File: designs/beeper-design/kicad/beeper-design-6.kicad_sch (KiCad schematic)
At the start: 23 parts, among them U3 BQ51003YFPR, U5 FH19C-6S-0.5SH(10)

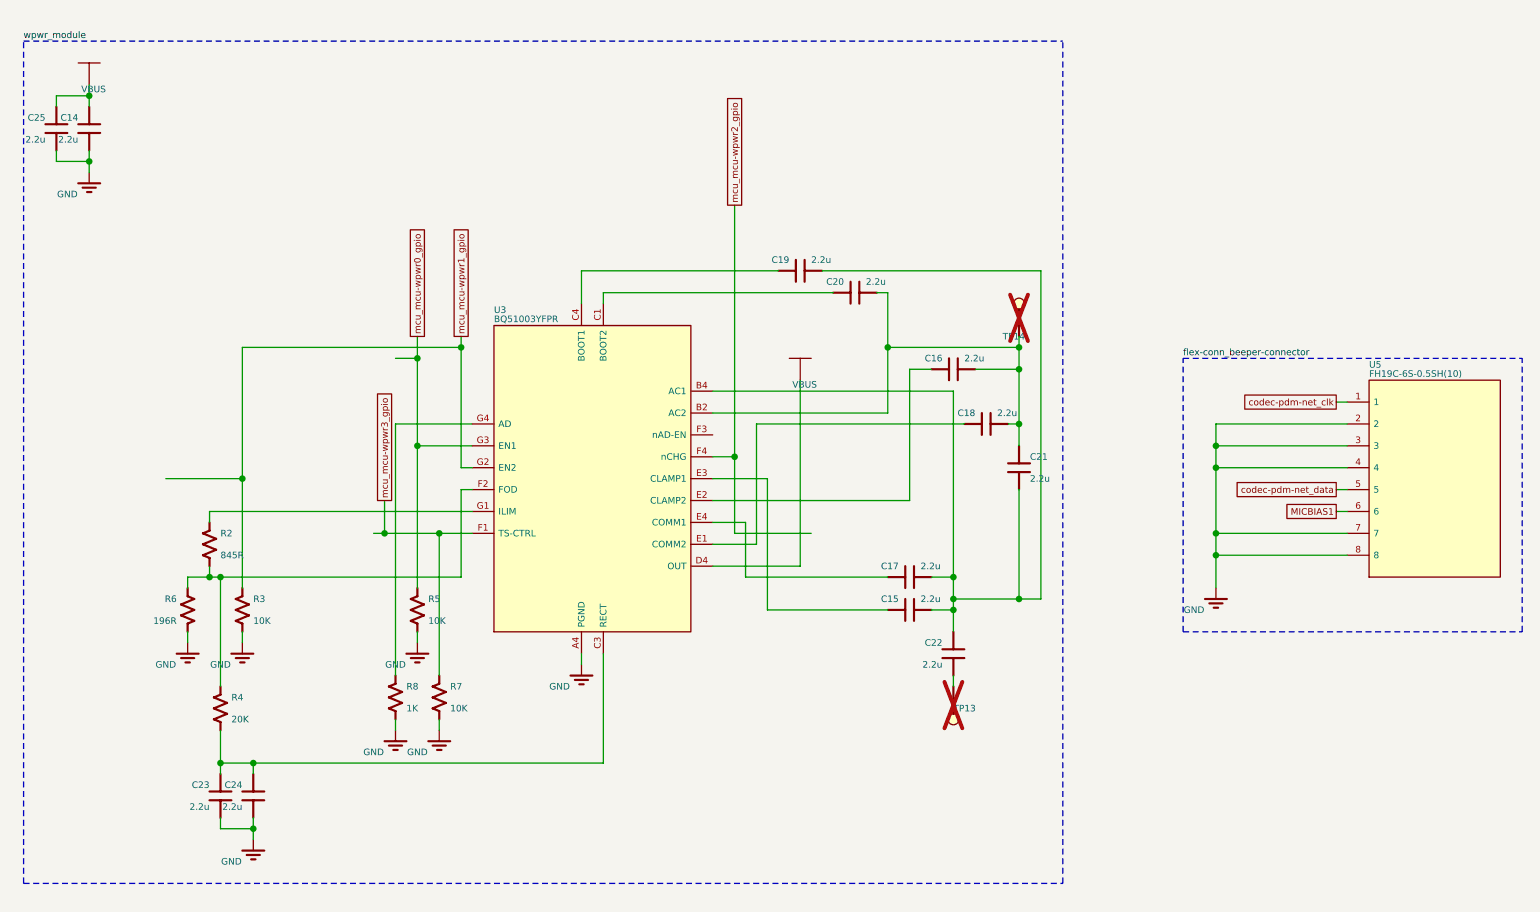
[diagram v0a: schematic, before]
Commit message: new export
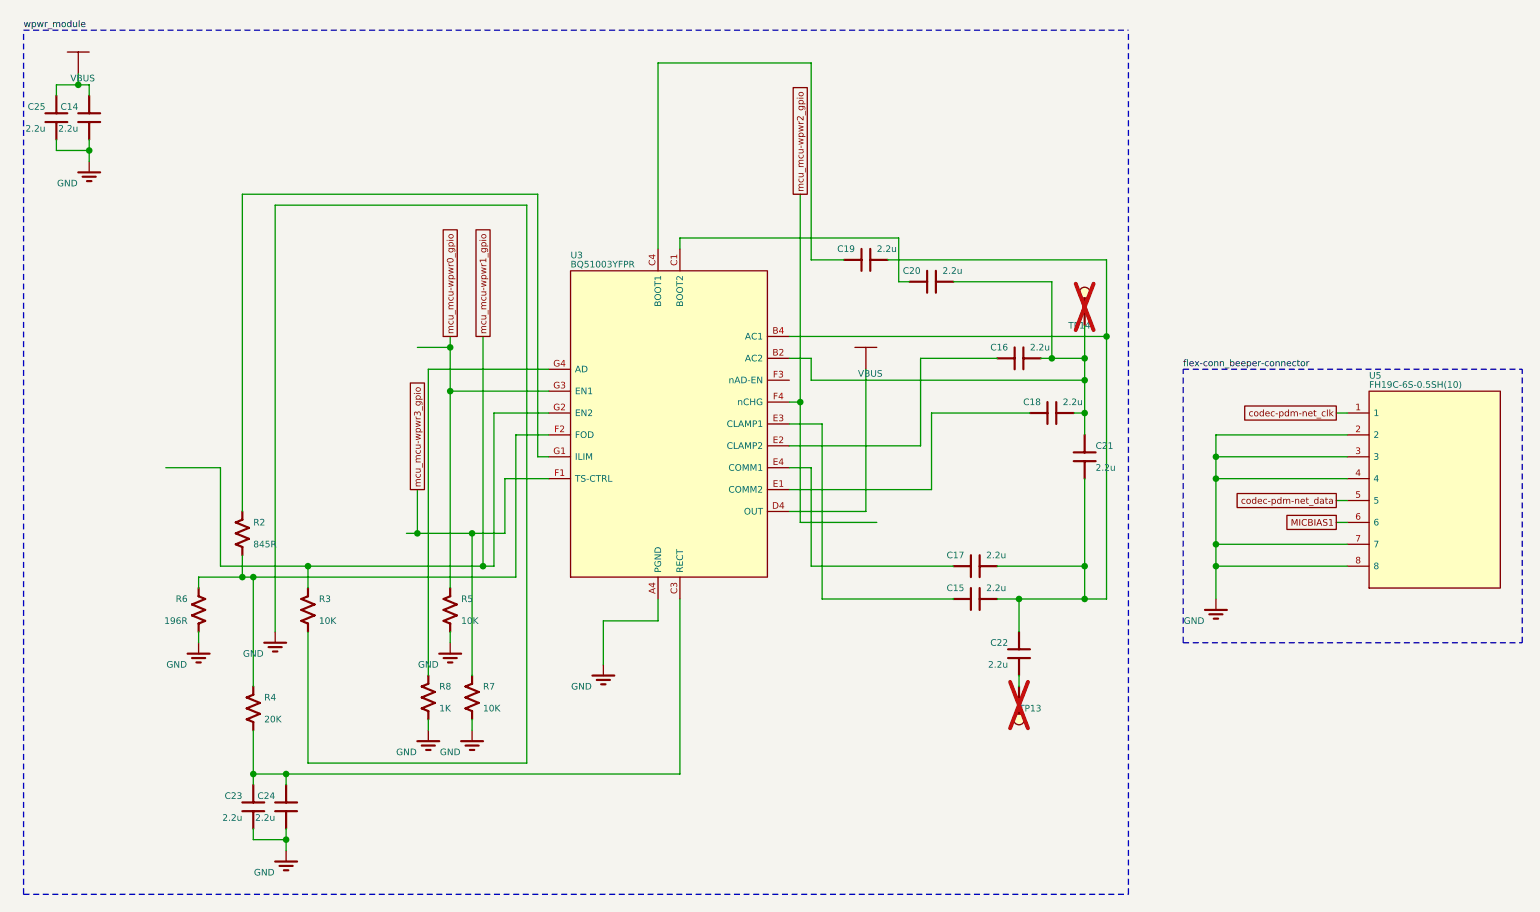
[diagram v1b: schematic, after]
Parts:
- removed C14: 2.2u, beeper-design:Pkg0201_2, symbol C335106
- removed C15: 2.2u, beeper-design:Pkg0201_51, symbol C335106_35
- removed C16: 2.2u, beeper-design:Pkg0201_12, symbol C335106_10
- removed C17: 2.2u, beeper-design:Pkg0201_25, symbol C335106_18
- removed C18: 2.2u, beeper-design:Pkg0201_37, symbol C335106_26
- removed C19: 2.2u, beeper-design:Pkg0201_49, symbol C335106_33
- removed C20: 2.2u, beeper-design:Pkg0201_10, symbol C335106_8
- removed C21: 2.2u, beeper-design:Pkg0201_23, symbol C335106_16
- removed C22: 2.2u, beeper-design:Pkg0201_35, symbol C335106_25
- removed C23: 2.2u, beeper-design:Pkg0201_48, symbol C335106_32
- removed C24: 2.2u, beeper-design:Pkg0201_7, symbol C335106_5
- removed C25: 2.2u, beeper-design:Pkg0201_22, symbol C335106_15
- removed R2: 845R, beeper-design:Pkg0201_15, symbol my_resistor_1
- removed R4: 20K, beeper-design:Pkg0201_41, symbol my_resistor_10
- removed R7: 10K, beeper-design:Pkg0201_26, symbol my_resistor_5
- removed R8: 1K, beeper-design:Pkg0201_38, symbol my_resistor_8
- added C14: 2.2u, beeper-design:Pkg0201, symbol C335106_35
- added C15: 2.2u, beeper-design:Pkg0201_50, symbol C335106_31
- added C16: 2.2u, beeper-design:Pkg0201_9, symbol C335106_7
- added C17: 2.2u, beeper-design:Pkg0201_22, symbol C335106_14
- added C18: 2.2u, beeper-design:Pkg0201_36, symbol C335106_22
- added C19: 2.2u, beeper-design:Pkg0201_49, symbol C335106_30
- added C20: 2.2u, beeper-design:Pkg0201_7, symbol C335106_5
- added C21: 2.2u, beeper-design:Pkg0201_20, symbol C335106_12
- added C22: 2.2u, beeper-design:Pkg0201_33, symbol C335106_20
- added C23: 2.2u, beeper-design:Pkg0201_48, symbol C335106_29
- added C24: 2.2u, beeper-design:Pkg0201_6, symbol C335106_4
- added C25: 2.2u, beeper-design:Pkg0201_18, symbol C335106_11
- added R2: 845R, beeper-design:Pkg0201_15, symbol my_resistor_3
- added R4: 20K, beeper-design:Pkg0201_40, symbol my_resistor_11
- added R7: 10K, beeper-design:Pkg0201_23, symbol my_resistor_6
- added R8: 1K, beeper-design:Pkg0201_38, symbol my_resistor_10
- R3: footprint beeper-design:Pkg0201_14 -> beeper-design:Pkg0201_10
- R5: footprint beeper-design:Pkg0201 -> beeper-design:Pkg0201_52
- R6: footprint beeper-design:Pkg0201_28 -> beeper-design:Pkg0201_27
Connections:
- net GND: now also C14.1, C23.1, C24.1, C25.1, R7.2, R8.2
- net VBUS: now also C14.2, C25.2
- net mcu_mcu-wpwr3_gpio: now also R7.1
- net at TP14.p, U3.B1 (AC2), U3.B2 (AC2): now also C16.1, C18.1, C20.1, C21.1
- net at U3.C1 (BOOT2): now also C20.2
- net at U3.C2 (RECT), U3.C3 (RECT): now also C23.2, C24.2, R4.2
- net at R6.1, U3.F2 (FOD): now also R2.2, R4.1
- net at U3.E1 (COMM2): now also C18.2
- net at U3.B3 (AC1), U3.B4 (AC1): now also C15.1, C17.1, C19.1, C21.2, C22.2
- net at U3.C4 (BOOT1): now also C19.2
- net at U3.E2 (CLAMP2): now also C16.2
- net at U3.E3 (CLAMP1): now also C15.2
- net at U3.E4 (COMM1): now also C17.2
- net at U3.G1 (ILIM): now also R2.1
- net at U3.G4 (AD): now also R8.1
- net at TP13.p: now also C22.1

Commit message: reasonble export
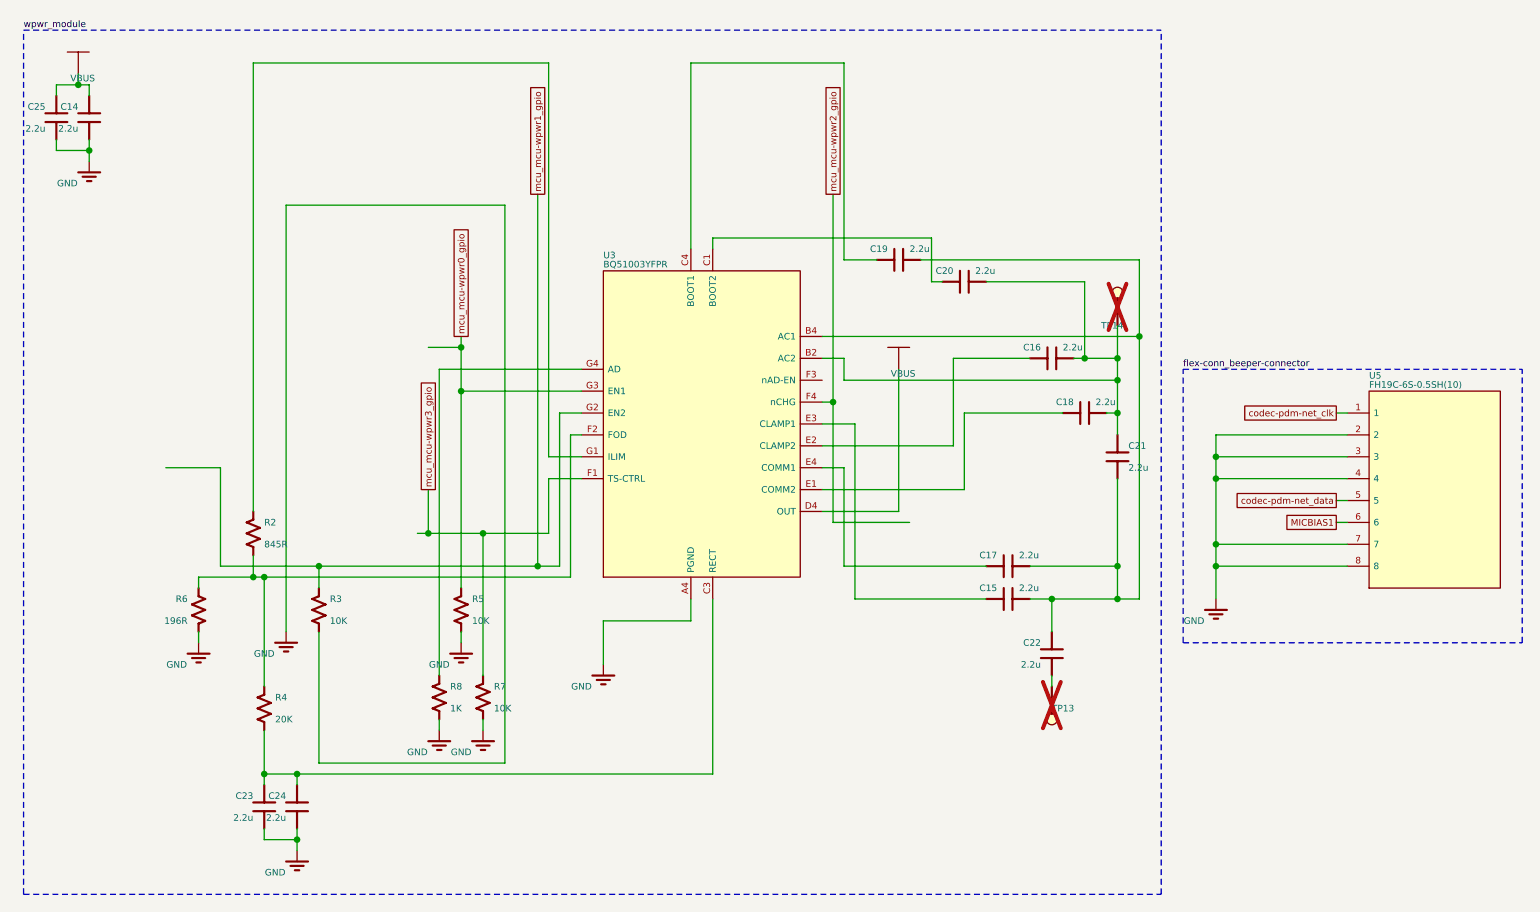
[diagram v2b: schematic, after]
